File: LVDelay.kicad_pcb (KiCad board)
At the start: 4 copper layers, 100.1 x 102.4 mm, 2 parts, among them J1 Conn_02x16, J2 Conn_02x16

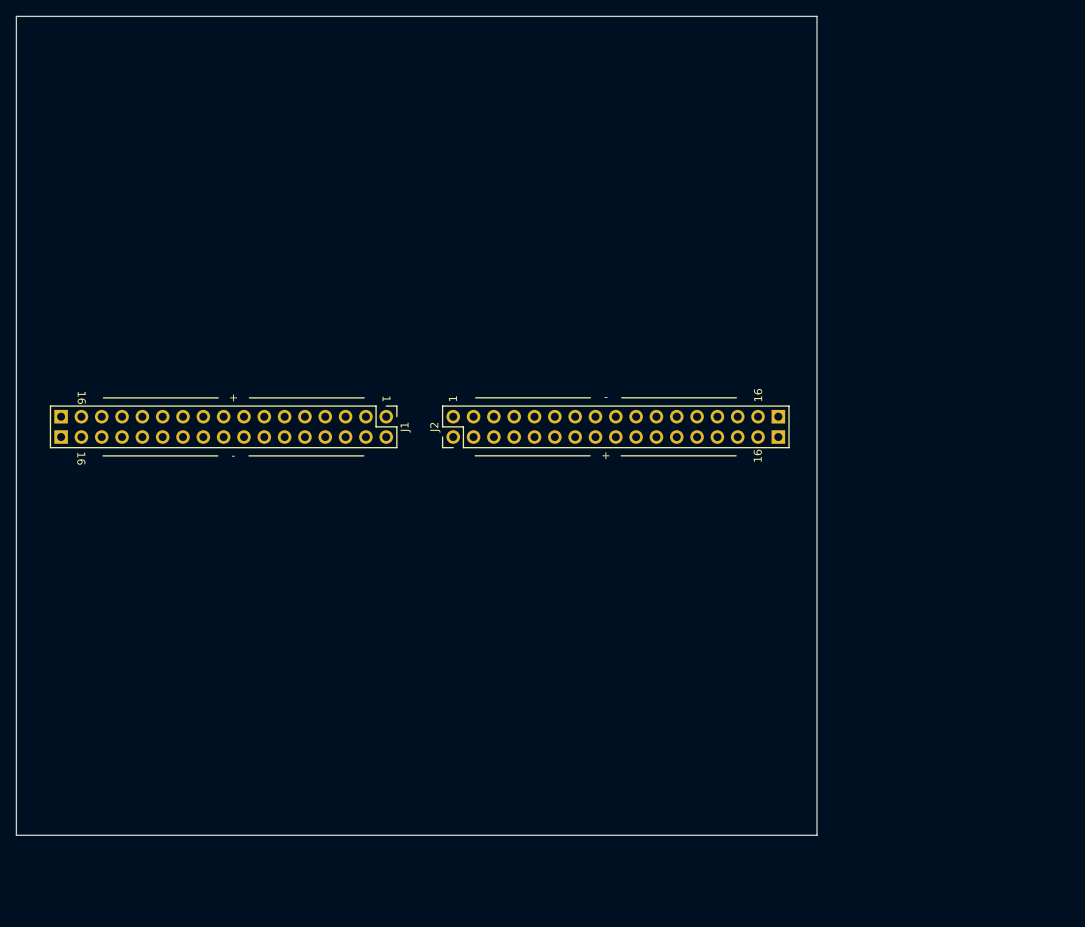
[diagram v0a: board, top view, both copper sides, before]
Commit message: Routing v1
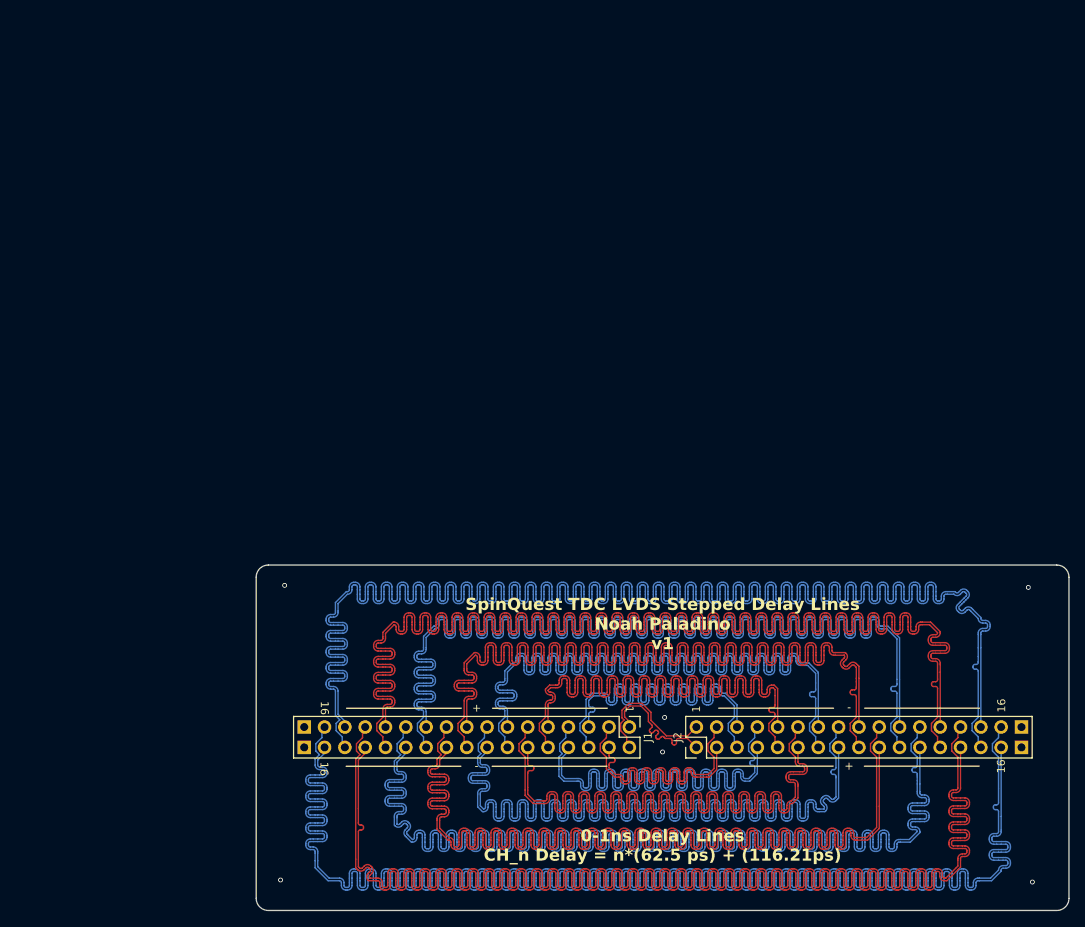
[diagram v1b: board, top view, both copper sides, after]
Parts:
- moved J1 49.3 mm to (96.9, 71.1)
- moved J2 49.3 mm to (105.3, 73.6)
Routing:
- net /Ch15+: track 0.00 -> 300.4 mm
- net /Ch15-: track 0.00 -> 300.4 mm
- net /Ch14+: track 0.00 -> 281.6 mm
- net /Ch14-: track 0.00 -> 281.6 mm
- net /Ch13+: track 0.00 -> 262.8 mm
- net /Ch13-: track 0.00 -> 262.8 mm
- net /Ch12-: track 0.00 -> 243.8 mm
- net /Ch12+: track 0.00 -> 243.8 mm
- net /Ch11-: track 0.00 -> 225.0 mm
- net /Ch11+: track 0.00 -> 224.9 mm
- net /Ch10-: track 0.00 -> 206.2 mm
- net /Ch10+: track 0.00 -> 206.2 mm
- net /Ch9+: track 0.00 -> 187.4 mm
- net /Ch9-: track 0.00 -> 186.5 mm
- net /Ch8-: track 0.00 -> 168.5 mm
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- added copper zone on In1.Cu, net GND
- added copper zone on In2.Cu, net GND
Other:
- board size 100.1 x 102.4 mm -> 101.6 x 43.2 mm
- board text added: "0-1ns Delay Lines CH_n Delay = n*(62.5 ps) + (116.21ps)"
- board text added: "SpinQuest TDC LVDS Stepped Delay Lines Noah Paladino v1"
